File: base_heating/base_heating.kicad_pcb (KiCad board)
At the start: 2 copper layers, 40.7 x 47.4 mm, 17 parts, among them J1 Moat_Bus_16, J10 1wireConn, J2 Moat_Bus_wire, J3 SCLK, J4 SDA, J5 3V3, J6 GND, J7 Conn_01x05, J8 S1, J9 S2, Q1 2N7002, Q2 2N7002

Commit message: Fix symbols
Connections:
- net GND renamed Net-(J1-GND)
- J1 pad 1: Net-(J1-Pad1) -> unconnected-(J1-KNX)
- J1 pad 2: Net-(J1-Pad2) -> unconnected-(J1-GND_KNX)
- J2 pad 13: (no net) -> unconnected-(J2-Bus4_12)
- J2 pad 15: (no net) -> unconnected-(J2-TxD)
- J2 pad 17: (no net) -> unconnected-(J2-RxD)
- J2 pad 6: (no net) -> unconnected-(J2-TxD3)
- J2 pad 8: (no net) -> unconnected-(J2-RxD3)
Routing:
- net unconnected-(J1-KNX): track 0.00 -> 8.25 mm
- net Net-(J1-Pad1): track 8.25 -> 0.00 mm
- net unconnected-(J1-GND_KNX): track 0.00 -> 7.10 mm
- net Net-(J1-Pad2): track 7.10 -> 0.00 mm

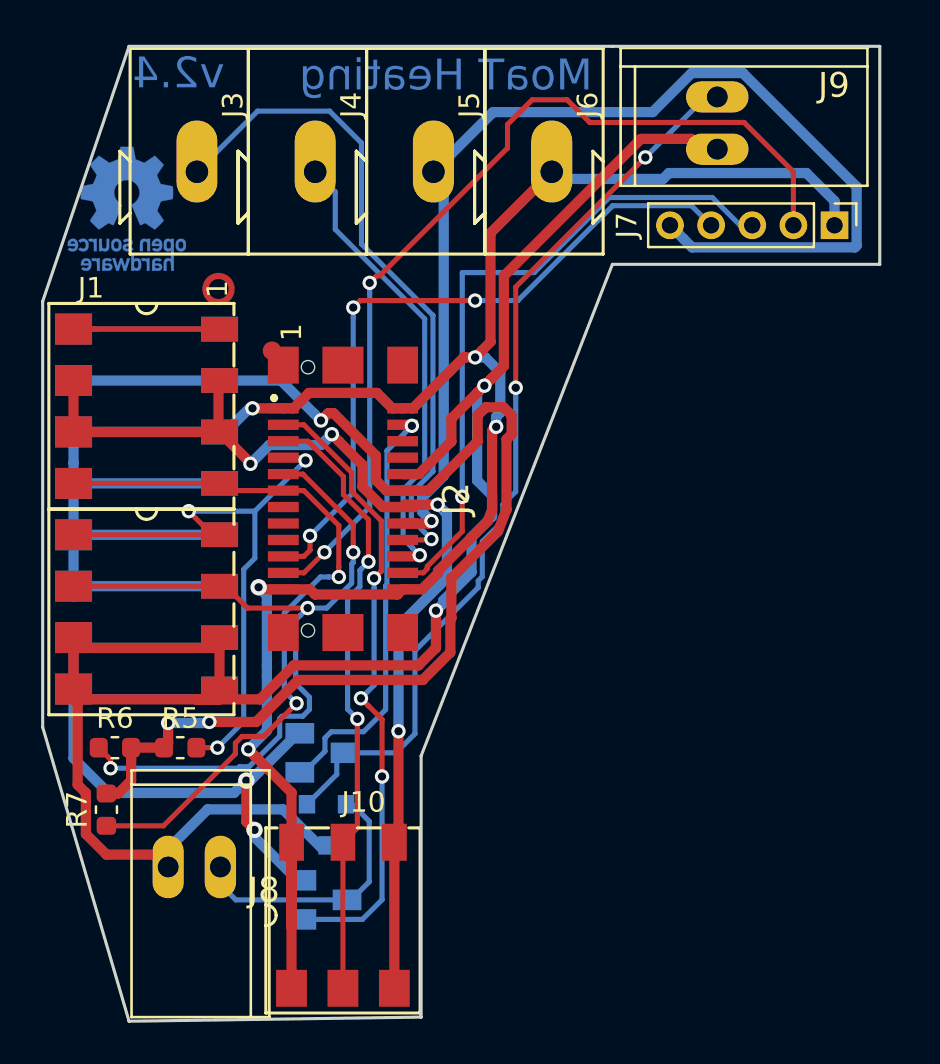
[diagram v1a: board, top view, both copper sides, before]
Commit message: *sigh*
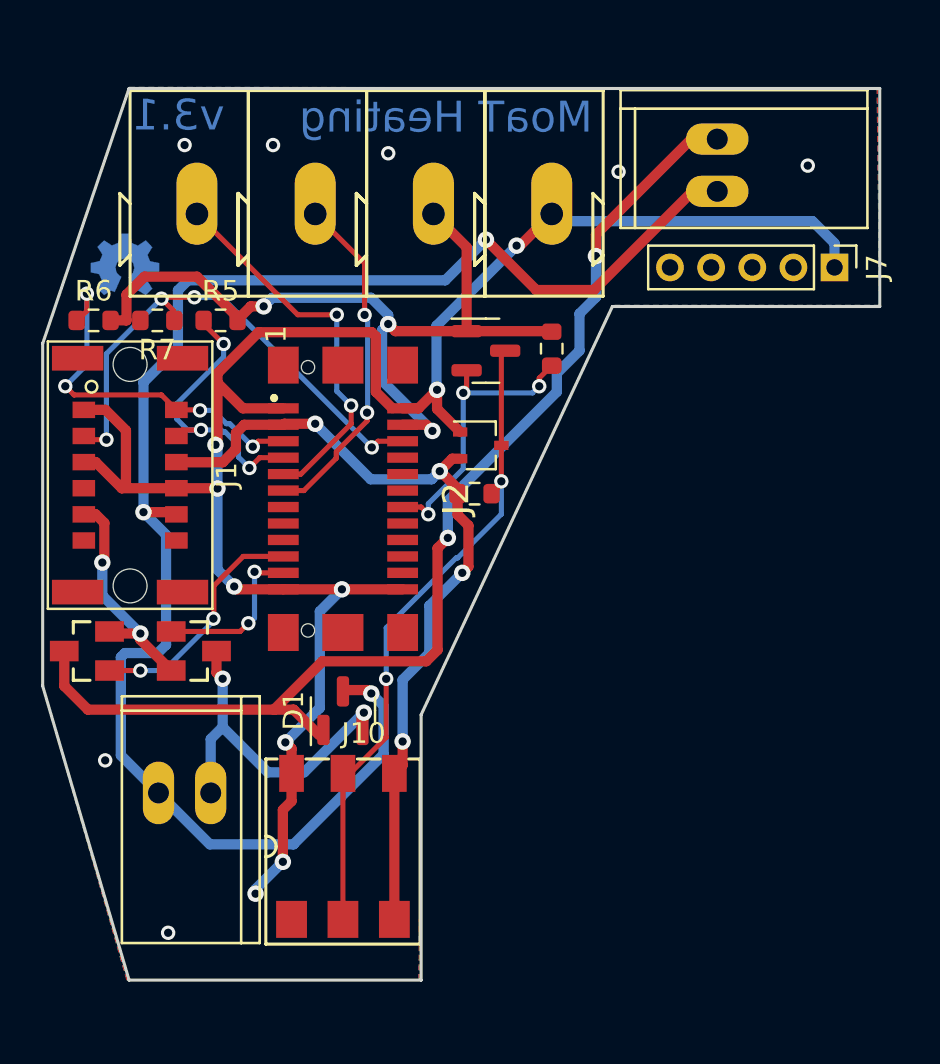
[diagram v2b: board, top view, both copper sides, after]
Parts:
- removed REF**: OSHW-Logo_5.7x6mm_Copper, Symbol:OSHW-Logo_5.7x6mm_Copper
- added D2: BAT54SW, Package_TO_SOT_SMD:SOT-323_SC-70, F.Cu at (40.6, 48.9)
- added G***: LOGO, localstuff:OSHW Logo 3mm Cu, B.Cu at (23.3, 40.1)
- added Q3: 2N7002, Package_TO_SOT_SMD:SOT-23, F.Cu at (40.9, 44.3)
- added R1: 10k, Resistor_SMD:R_0603_1608Metric, F.Cu at (44.0, 44.2)
- added R2: 10k, Resistor_SMD:R_0603_1608Metric, F.Cu at (40.3, 51.2)
- D1, Q1, Q2: moved to F.Cu
- J1: value Moat_Bus_16 -> Moat_Bus_12; footprint localstuff:Moat_16_2side -> localstuff:MoaT_12_Pin_V
- moved R7 23.9 mm to (24.9, 42.8), turned to 180 degrees
- moved R5 20.9 mm to (27.9, 42.8)
- moved R6 20.8 mm to (21.8, 42.8)
- moved Q1 13.7 mm to (26.6, 58.9), turned to -90 degrees
- moved Q2 12.5 mm to (21.4, 58.9)
- moved D1 5.61 mm to (33.9, 61.8), turned to 90 degrees
- moved J8 3.63 mm to (26.2, 65.8)
- moved J10 3.35 mm to (33.9, 68.4)
- moved J1 2.13 mm to (23.6, 50.4)
- moved J9 2.05 mm to (52.1, 35.3)
- moved J3 2.05 mm to (26.8, 37.7)
- moved J4 2.05 mm to (32.5, 37.7)
- moved J5 2.05 mm to (38.3, 37.7)
- moved J6 2.05 mm to (44.0, 37.7)
- moved J7 2.05 mm to (57.8, 40.3)
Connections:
- net Net-(Q1-D) renamed /S1G
- net Net-(Q2-D) renamed /S2G
- J1 pad 1: unconnected-(J1-KNX) -> GND
- J1 pad 10: Net-(J1-GND) -> +24V
- J1 pad 11: Net-(J1-Bus1_12) -> unconnected-(J1-KNX)
- J1 pad 12: Net-(J1-GND) -> unconnected-(J1-GND_KNX)
- J1 pad 2: unconnected-(J1-GND_KNX) -> /Bus1
- J1 pad 3: +5V -> /Bus2
- J1 pad 4: +12V -> /Bus3
- J1 pad 5: +5V -> GND
- J1 pad 6: Net-(J1-GND) -> +5V
- J1 pad 7: Net-(J1-Bus3_12) -> unconnected-(J1-12V)
- J1 pad 8: Net-(J1-GND) -> GND
- J1 pad 9: Net-(J1-Bus2_12) -> GNDPWR
- J10 pad 1: Net-(J1-GND) -> GND
- J10 pad 2: Net-(J10-1wire) -> /1wire_5
- J2 pad 1: Net-(J1-GND) -> GND
- J2 pad 10: +24V -> unconnected-(J2-Rx)
- J2 pad 11: Net-(J1-Bus3_12) -> /SDa
- J2 pad 12: +12V -> unconnected-(J2-Tx)
- J2 pad 14: +5V -> /1wire_3
- J2 pad 16: Net-(J2-3V3) -> unconnected-(J2-T4)
- J2 pad 18: Net-(J2-CLK) -> /T3
- J2 pad 19: Net-(J2-T3) -> /S2
- J2 pad 2: Net-(J1-GND) -> GND
- J2 pad 20: Net-(J2-DAT) -> /T2
- J2 pad 21: Net-(J2-T1) -> /S1
- J2 pad 22: Net-(J2-T2) -> /T1
- J2 pad 23: Net-(J1-GND) -> GND
- J2 pad 24: Net-(J1-GND) -> GND
- J2 pad 3: /S1 -> +5V
- J2 pad 4: /S2 -> +3V3
- J2 pad 5: Net-(J10-1wire) -> /Bus1
- J2 pad 6: unconnected-(J2-TxD3) -> /Bus2
- J2 pad 7: Net-(J1-Bus2_12) -> /Bus3
- J2 pad 9: Net-(J1-Bus1_12) -> /SCl
- J3 pad 1: Net-(J2-CLK) -> /SCl
- J4 pad 1: Net-(J2-DAT) -> /SDa
- J5 pad 1: Net-(J2-3V3) -> +3V3
- J6 pad 1: Net-(J1-GND) -> GND
- J7 pad 1: Net-(J1-GND) -> GND
- J7 pad 2: Net-(J2-T1) -> unconnected-(J7-Pin_2)
- J7 pad 3: Net-(J2-T2) -> unconnected-(J7-Pin_3)
- J7 pad 4: Net-(J2-T3) -> unconnected-(J7-Pin_4)
- J7 pad 5: Net-(J2-3V3) -> unconnected-(J7-Pin_5)
- R5 pad 1: +12V -> /Bus3
- R5 pad 2: Net-(J1-Bus2_12) -> +3V3
- R6 pad 1: Net-(J1-Bus1_12) -> /Bus1
- R6 pad 2: +12V -> +3V3
- R7 pad 1: Net-(J1-Bus3_12) -> /Bus2
- R7 pad 2: +12V -> +3V3
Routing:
- net Net-(J1-GND): track 124.0 -> 0.00 mm, vias 5 -> 0
- net GND: track 0.00 -> 94.9 mm, vias 0 -> 16
- net +12V: track 60.8 -> 0.00 mm, vias 3 -> 0
- net Net-(J2-3V3): track 56.5 -> 0.00 mm, vias 1 -> 0
- net Net-(J2-T1): track 45.4 -> 0.00 mm, vias 2 -> 0
- net Net-(J1-Bus1_12): track 39.8 -> 0.00 mm, vias 3 -> 0
- net +3V3: track 0.00 -> 39.5 mm, vias 0 -> 3
- net Net-(J1-Bus3_12): track 37.4 -> 0.00 mm, vias 2 -> 0
- net Net-(J2-T3): track 33.9 -> 0.00 mm, vias 3 -> 0
- net Net-(J2-CLK): track 32.8 -> 0.00 mm, vias 1 -> 0
- net Net-(J2-T2): track 32.6 -> 0.00 mm, vias 1 -> 0
- net /1wire_5: track 0.00 -> 32.0 mm, vias 0 -> 2
- net Net-(J1-Bus2_12): track 30.2 -> 0.00 mm, vias 3 -> 0
- net Net-(J10-1wire): track 29.9 -> 0.00 mm, vias 2 -> 0
- net GNDPWR: track 38.6 -> 11.2 mm
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- added copper zone on B.Cu, net GND
- added copper zone on F.Cu, net GND
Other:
- board size 40.7 x 47.4 mm -> 40.7 x 43.3 mm
- board text added: "v3.1"
- board text removed: "v2.4"
